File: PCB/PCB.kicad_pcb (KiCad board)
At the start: 2 copper layers, 228 x 147.8 mm, 20 parts, among them SW1 SW4_Push, SW10 SW2_Push, SW11 SW3_Push, SW2 SW5_Push, SW3 RotaryEncoder_Switch, SW4 RotaryEncoder_Switch, SW5 SW6_Push, SW6 SW7_Push, SW7 SW_Push-Mode0, SW8 SW_Push-Mode1, SW9 SW1_Push, U4 ER_OLEDM0.91_1x-I2C, U5 MOUDLE-SEEEDUINO-XIAO

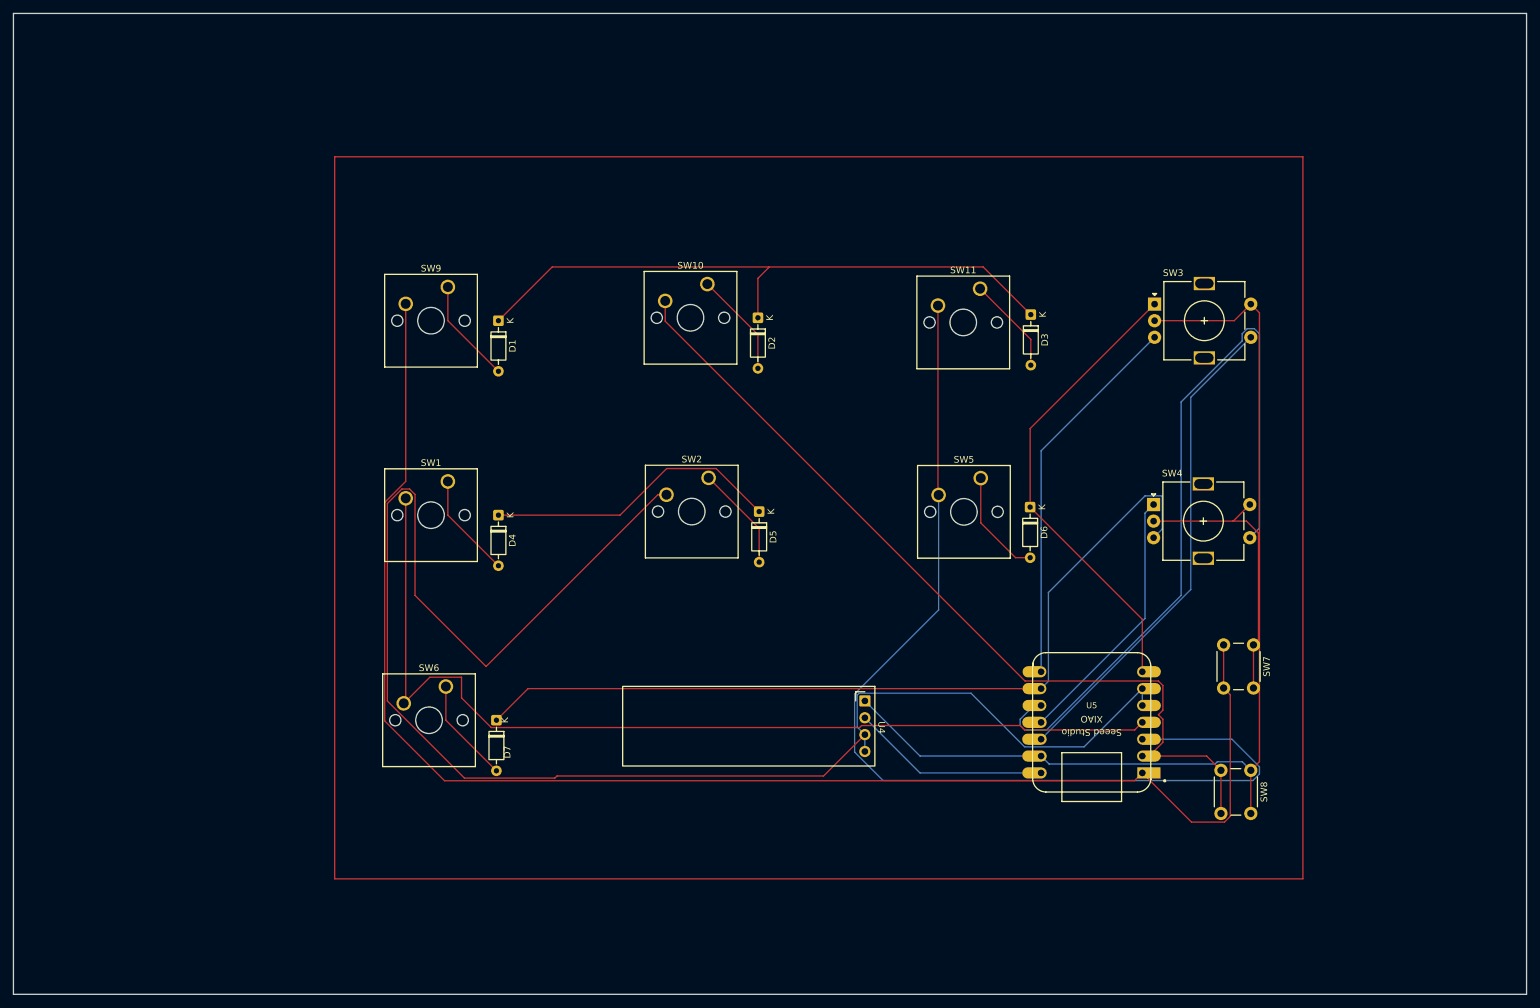
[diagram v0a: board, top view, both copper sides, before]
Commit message: Finalize PCB and manufacturing files
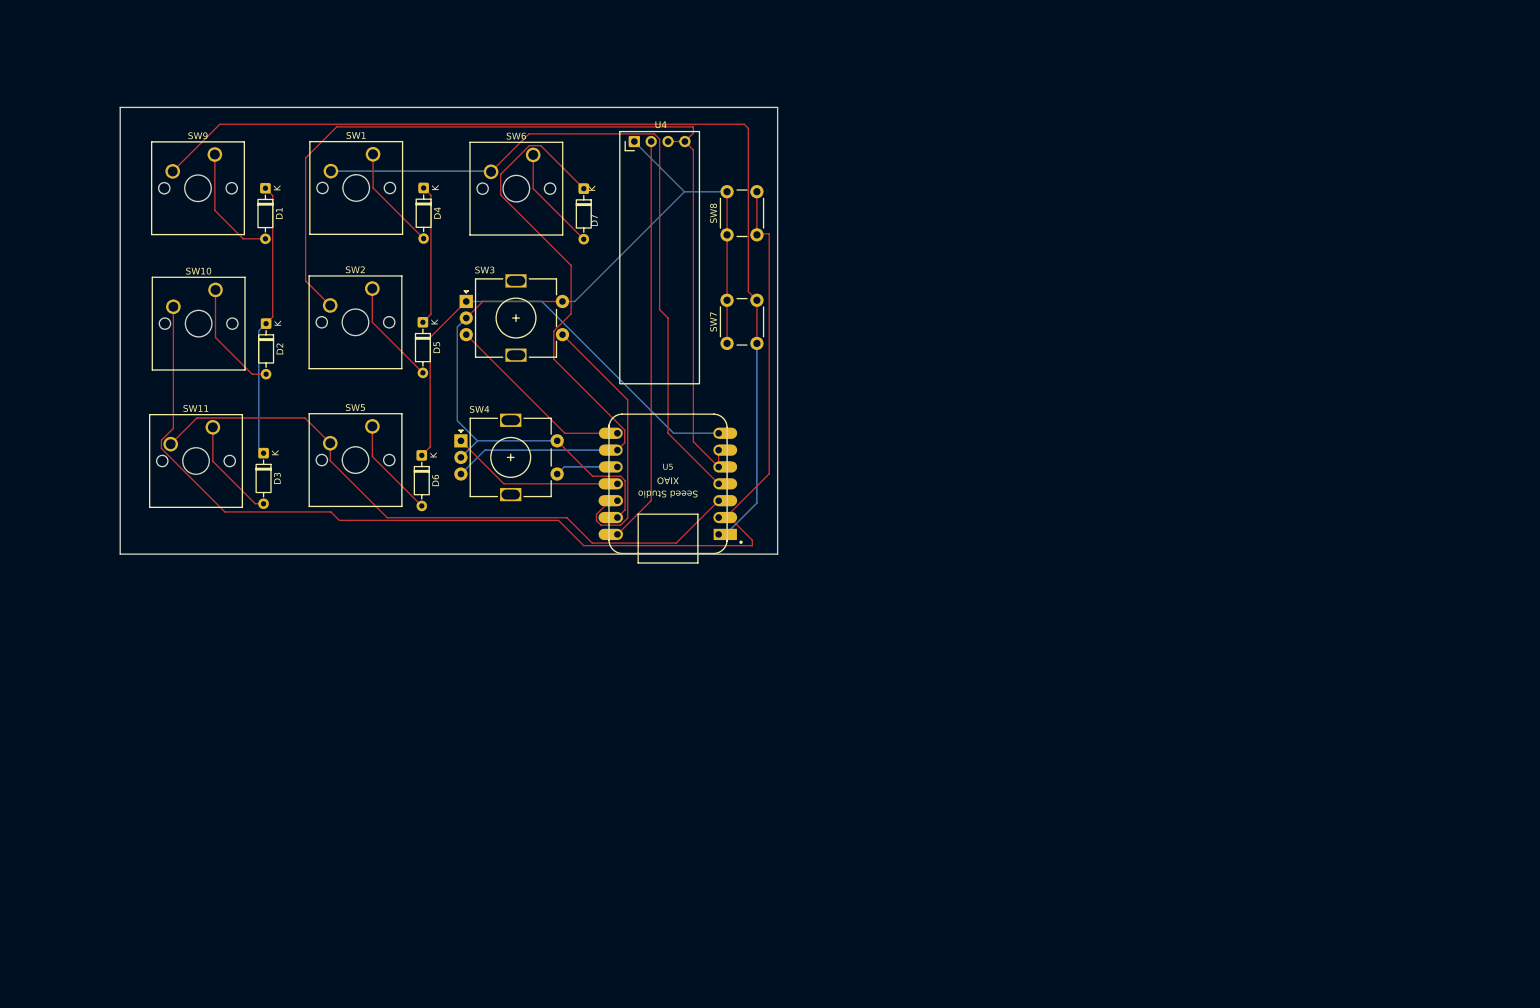
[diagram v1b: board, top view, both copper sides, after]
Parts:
- moved D3 117.5 mm to (81.3, 100.4)
- moved SW11 117.5 mm to (73.7, 96.5)
- moved SW8 112.9 mm to (151.1, 67.5), turned to 90 degrees
- moved SW4 104.8 mm to (111.0, 98.5)
- moved SW3 103.7 mm to (111.8, 77.5)
- moved D6 92.0 mm to (105.1, 100.7)
- moved SW5 92.0 mm to (97.7, 96.3)
- moved SW7 91.4 mm to (151.1, 83.8), turned to 90 degrees
- moved U4 91.2 mm to (137.2, 53.4), turned to 0 degrees
- moved SW6 81.2 mm to (121.9, 55.4)
- moved D7 81.2 mm to (129.5, 60.5)
- moved D2 74.1 mm to (81.7, 80.8)
- moved SW10 74.1 mm to (74.0, 75.8)
- moved U5 73.3 mm to (142.2, 105.0)
- moved D5 58.1 mm to (105.3, 80.6)
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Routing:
- net Net-(U5-PA5_A9_D9_MISO): track 115.7 -> 9.52 mm
- net Net-(U4-SCL): track 244.5 -> 143.1 mm
- net Net-(U5-PA02_A0_D0): track 225.5 -> 154.6 mm
- net Net-(U4-GND): track 201.7 -> 135.3 mm
- net Net-(U5-PA10_A2_D2): track 156.2 -> 96.2 mm
- net Net-(D1-K): track 94.9 -> 41.5 mm
- net Net-(U5-PA4_A1_D1): track 134.0 -> 179.4 mm
- net Net-(U5-PA11_A3_D3): track 149.8 -> 107.9 mm
- net Net-(D7-K): track 129.0 -> 94.0 mm
- net Net-(U5-3V3): track 73.6 -> 42.1 mm
- net Net-(U4-VCC): track 30.0 -> 61.3 mm
- net Net-(U5-PB09_A7_D7_RX): track 57.5 -> 28.9 mm
- net Net-(D4-K): track 44.9 -> 21.2 mm
- net Net-(U5-PA6_A10_D10_MOSI): track 39.8 -> 26.3 mm
- net Net-(D6-K): track 70.2 -> 73.1 mm
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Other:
- board size 228 x 147.8 mm -> 99.1 x 67.3 mm
